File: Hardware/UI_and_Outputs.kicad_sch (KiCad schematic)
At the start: 8 parts

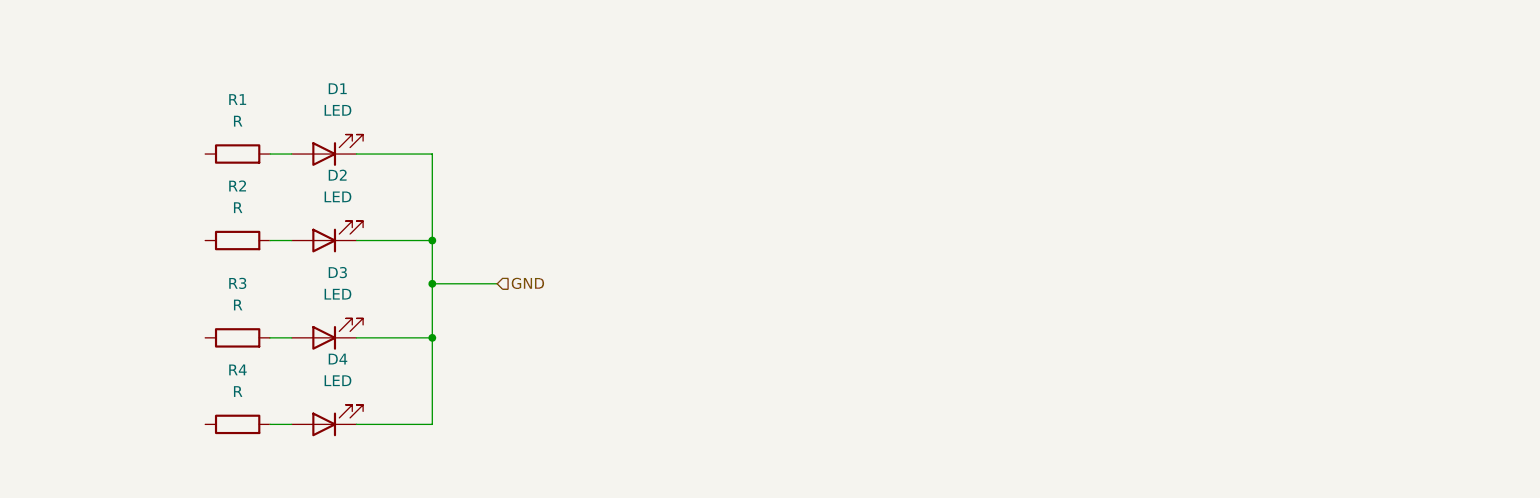
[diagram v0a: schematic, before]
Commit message: Major Updates to Schematic
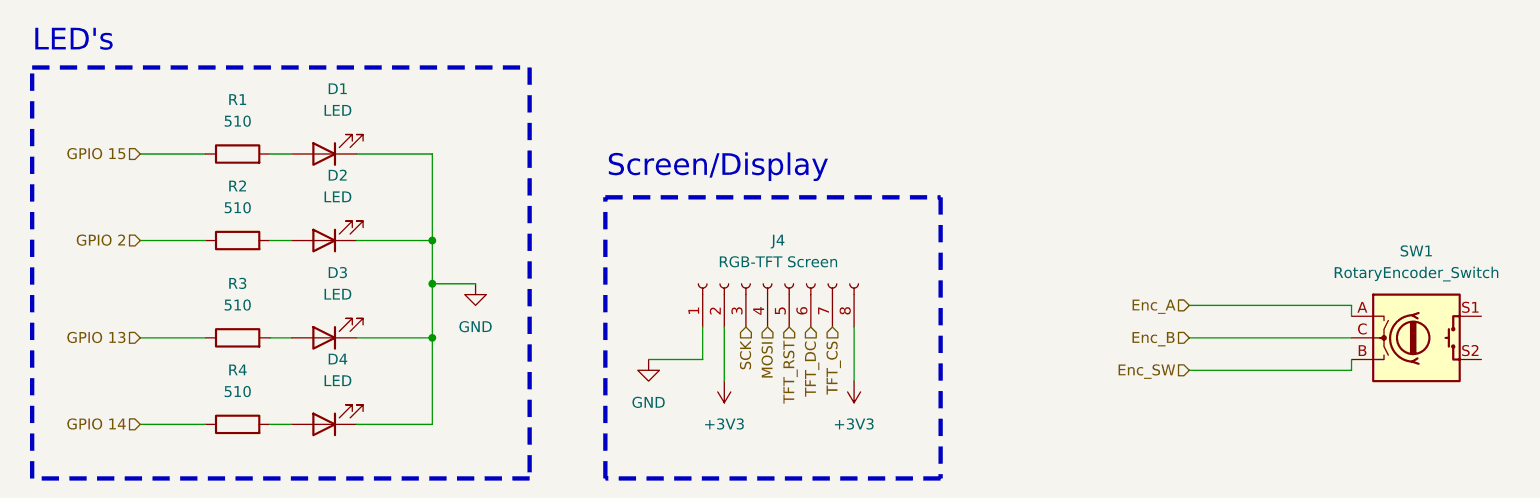
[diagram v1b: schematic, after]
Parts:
- added J4: RGB-TFT Screen, Custom_Screens:1.8_128x160_RGB-TFT, symbol Connector:Conn_01x08_Socket
- added SW1: RotaryEncoder_Switch, symbol Device:RotaryEncoder_Switch
- R1, R2, R3, R4: value R -> 510
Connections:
- net GND: now also J4.1 (Pin_1)
- net GPIO 2: now reaches R2.1
- net GPIO 13: now reaches R3.1
- net GPIO 15: now reaches R1.1
- net GPIO 14: now reaches R4.1
- new net +3V3: J4.2 (Pin_2), J4.8 (Pin_8)
- new net Enc_A: SW1.A
- new net Enc_B: SW1.C
- new net Enc_SW: SW1.B
- new net MOSI: J4.4 (Pin_4)
- new net SCK: J4.3 (Pin_3)
- new net TFT_CS: J4.7 (Pin_7)
- new net TFT_DC: J4.6 (Pin_6)
- new net TFT_RST: J4.5 (Pin_5)
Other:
- note added: "LED's"
- note added: "Screen/Display"
